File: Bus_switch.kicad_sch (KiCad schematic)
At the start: 8 parts, among them J3 Conn_01x04_Pin, U1 SN74CB3Q3384APW

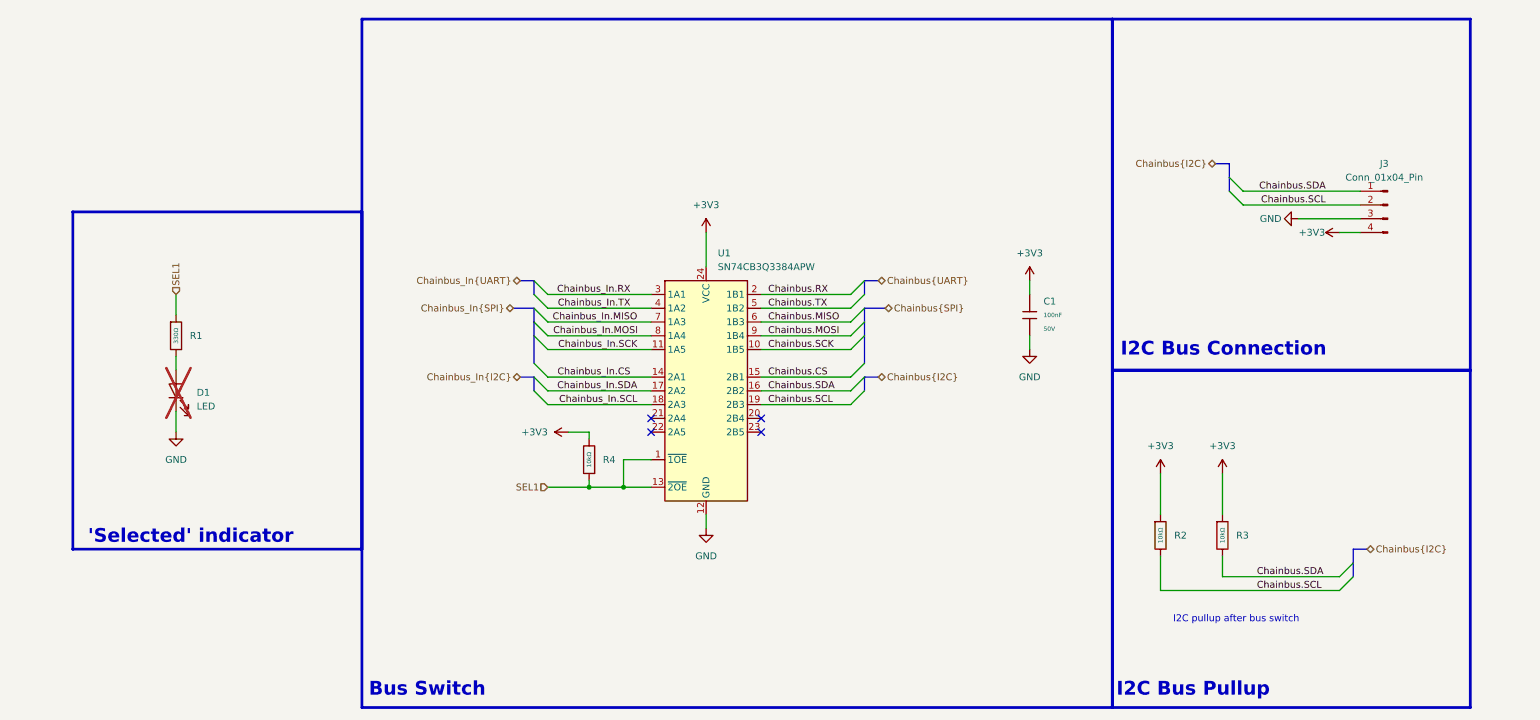
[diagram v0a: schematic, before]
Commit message: Updated footprints
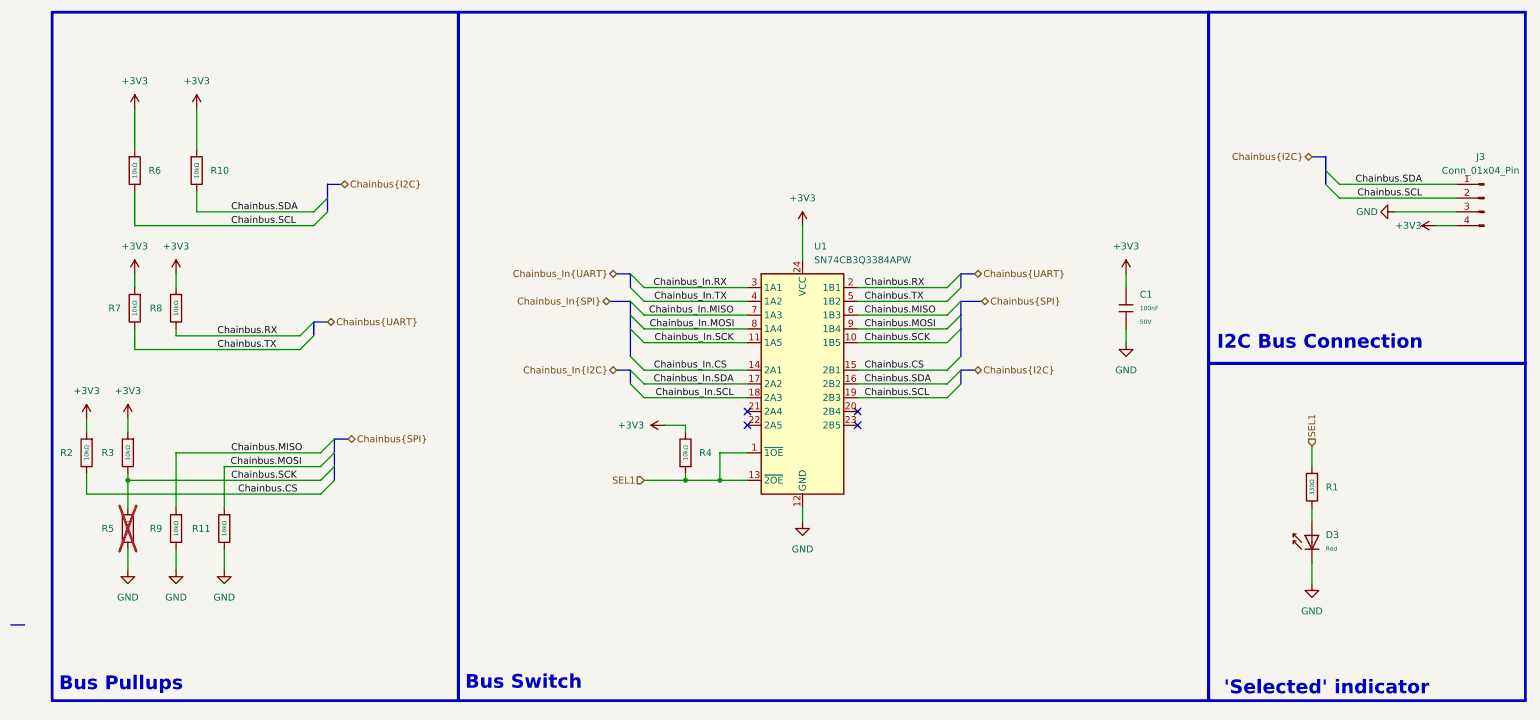
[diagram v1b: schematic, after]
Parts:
- removed D1: LED, LED_SMD:LED_0603_1608Metric, symbol Device:LED
- added D3: Red, PCM_JLCPCB:D_0603, symbol PCM_JLCPCB-Diodes:LED,0603,Red
- added R11, R2, R3, R5, R7, R8, R9: 10kΩ, PCM_JLCPCB:R_0402, symbol PCM_JLCPCB-Resistors:0402,10kΩ
- renumbered R3 to R10, R2 to R6
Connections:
- net +3V3: now also R2.1, R3.1, R7.1, R8.1
- net Chainbus.CS: now also R2.2
- net Chainbus.MISO: now also R9.1
- net Chainbus.MOSI: now also R11.1
- net Chainbus.RX: now also R8.2
- net Chainbus.SCK: now also R3.2, R5.1
- net Chainbus.TX: now also R7.2
- net GND: now also D3.1, R11.2, R5.2, R9.2
- net at R1.2: now also D3.2
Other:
- note added: "Bus Pullups"
- note removed: "I2C Bus Pullup"
- note removed: "I2C pullup after bus switch"
- moved on the sheet: C1, J3, R1, R10, R4, R6, U1
